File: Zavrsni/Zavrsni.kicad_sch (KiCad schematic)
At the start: 18 parts, among them J1 12V Source, J3 Output A, J4 Pin za Vin, J5 Conn_01x04, J6 Conn_02x19_Odd_Even, J7 Conn_02x19_Odd_Even, J8 Conn_01x06, U1 LM78M05_TO220, U2 L298N

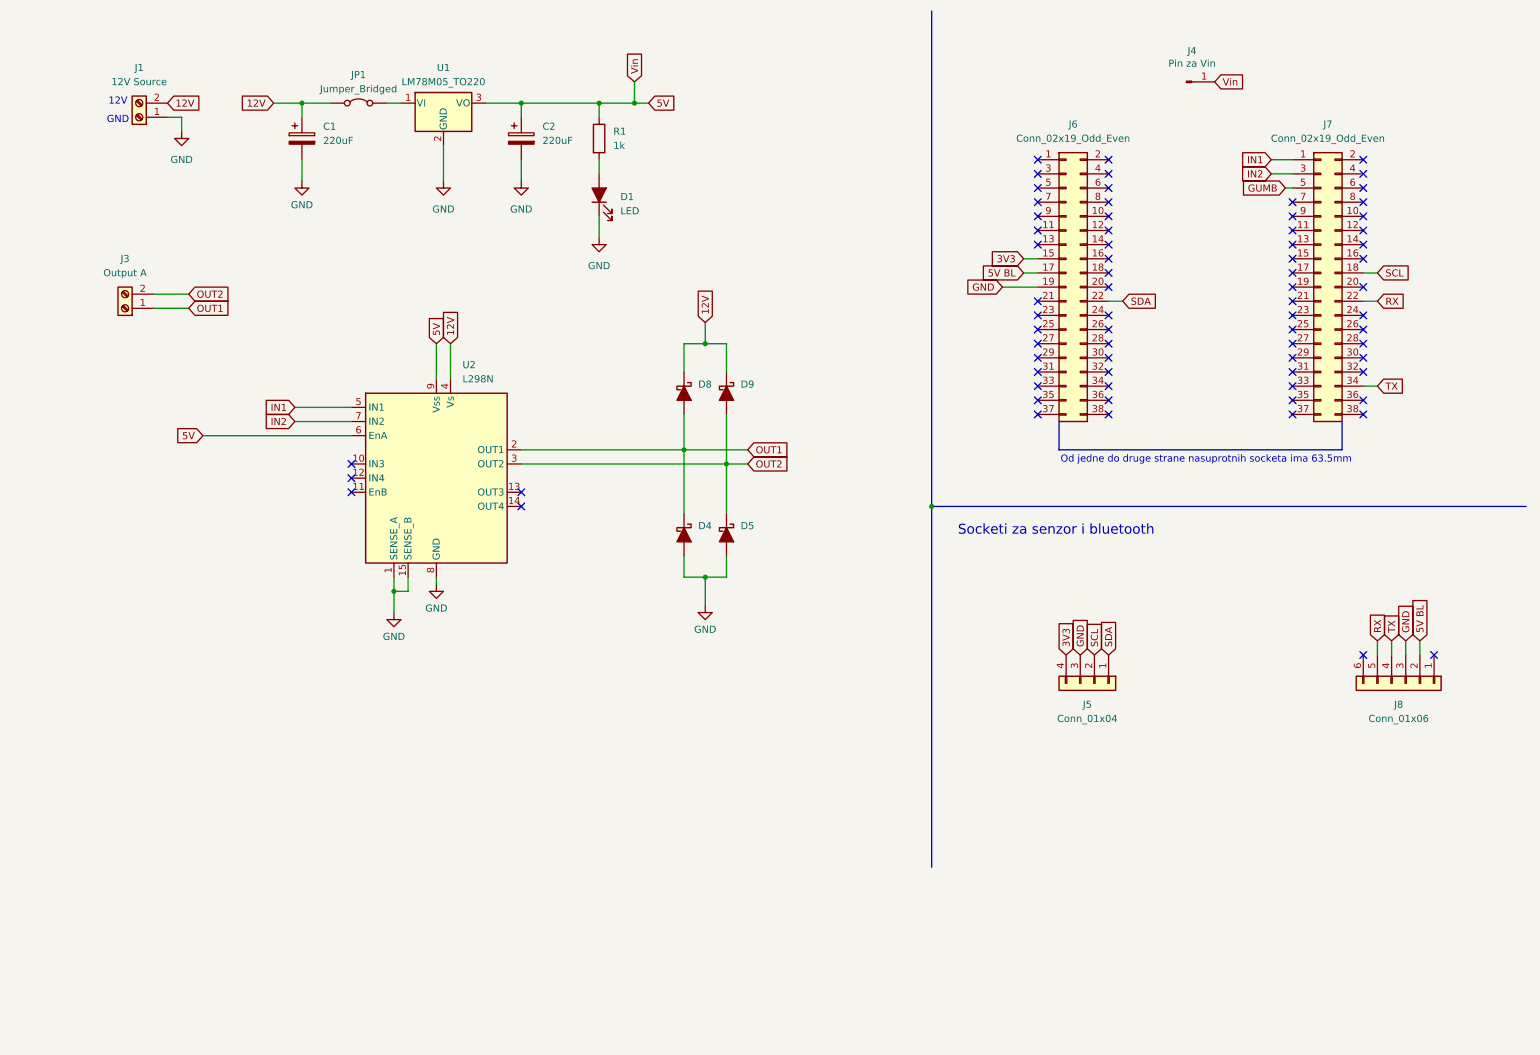
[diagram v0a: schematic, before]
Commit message: New
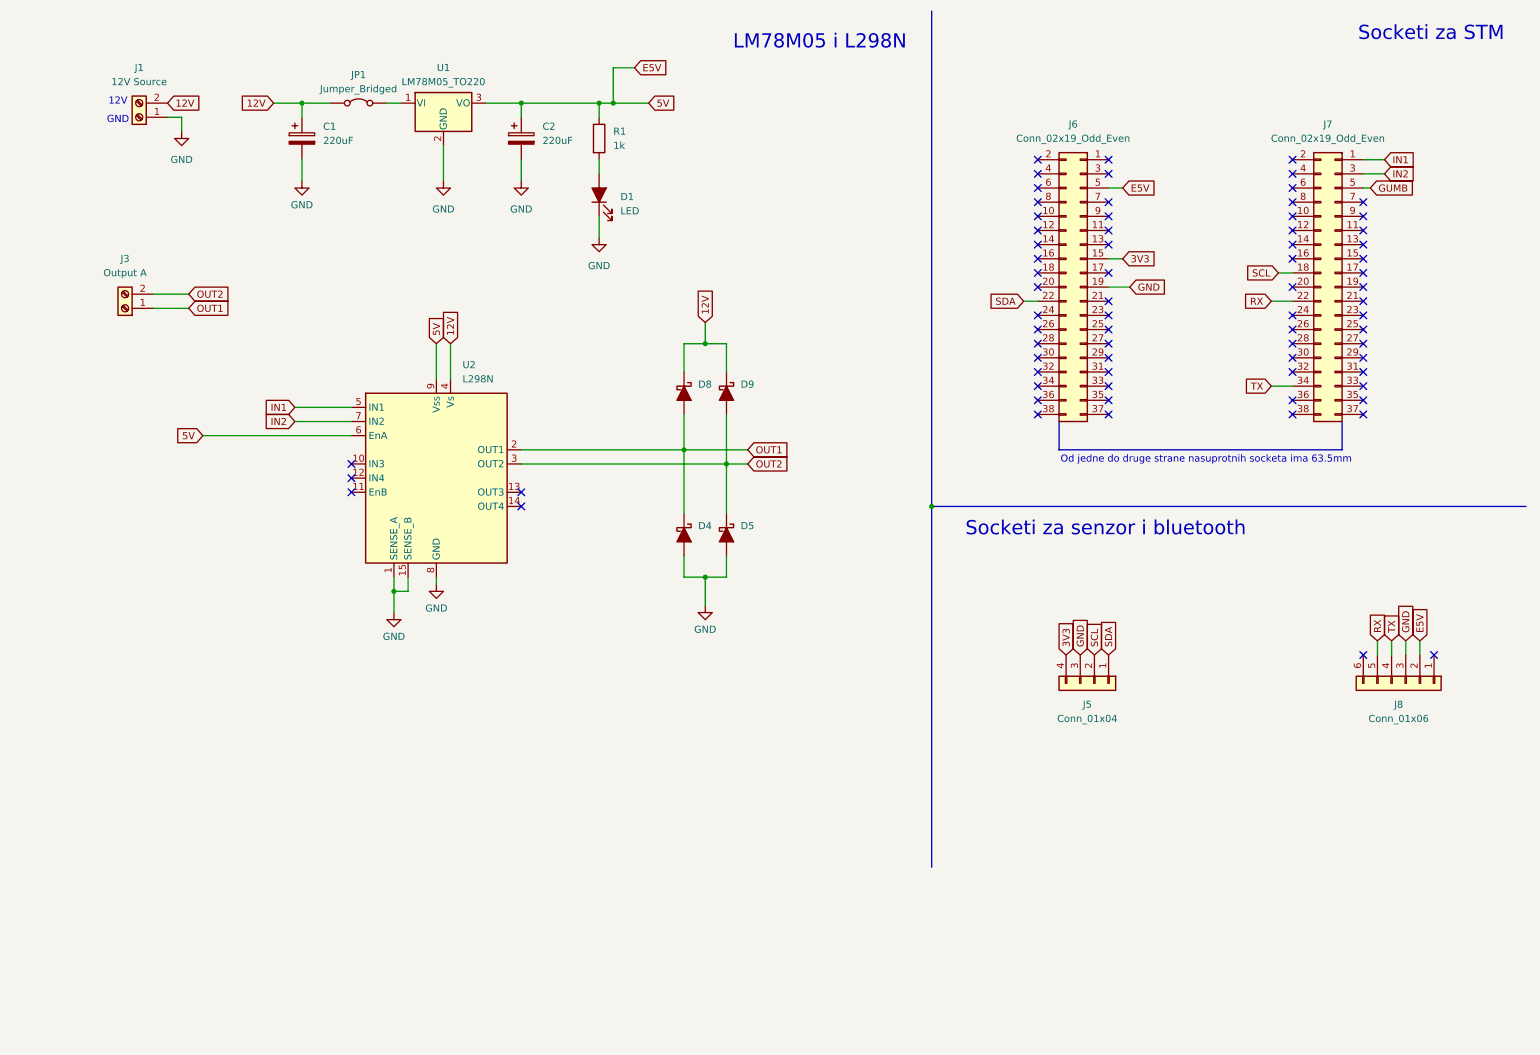
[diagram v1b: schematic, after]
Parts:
- removed J4: Pin za Vin, Connector_PinHeader_2.54mm:PinHeader_1x01_P2.54mm_Vertical, symbol Connector:Conn_01x01_Pin
- U1: Manufacturer (none) -> ONSEMI; Manufacturer part number (none) -> TO-220
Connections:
- net 5V: now also J6.5 (Pin_5), J8.2 (Pin_2)
- net 5V BL: no longer names the net of J6.17 (Pin_17)
- net 5V BL: no longer J8.2 (Pin_2)
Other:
- note added: "LM78M05 i L298N"
- note added: "Socketi za STM"

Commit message: New
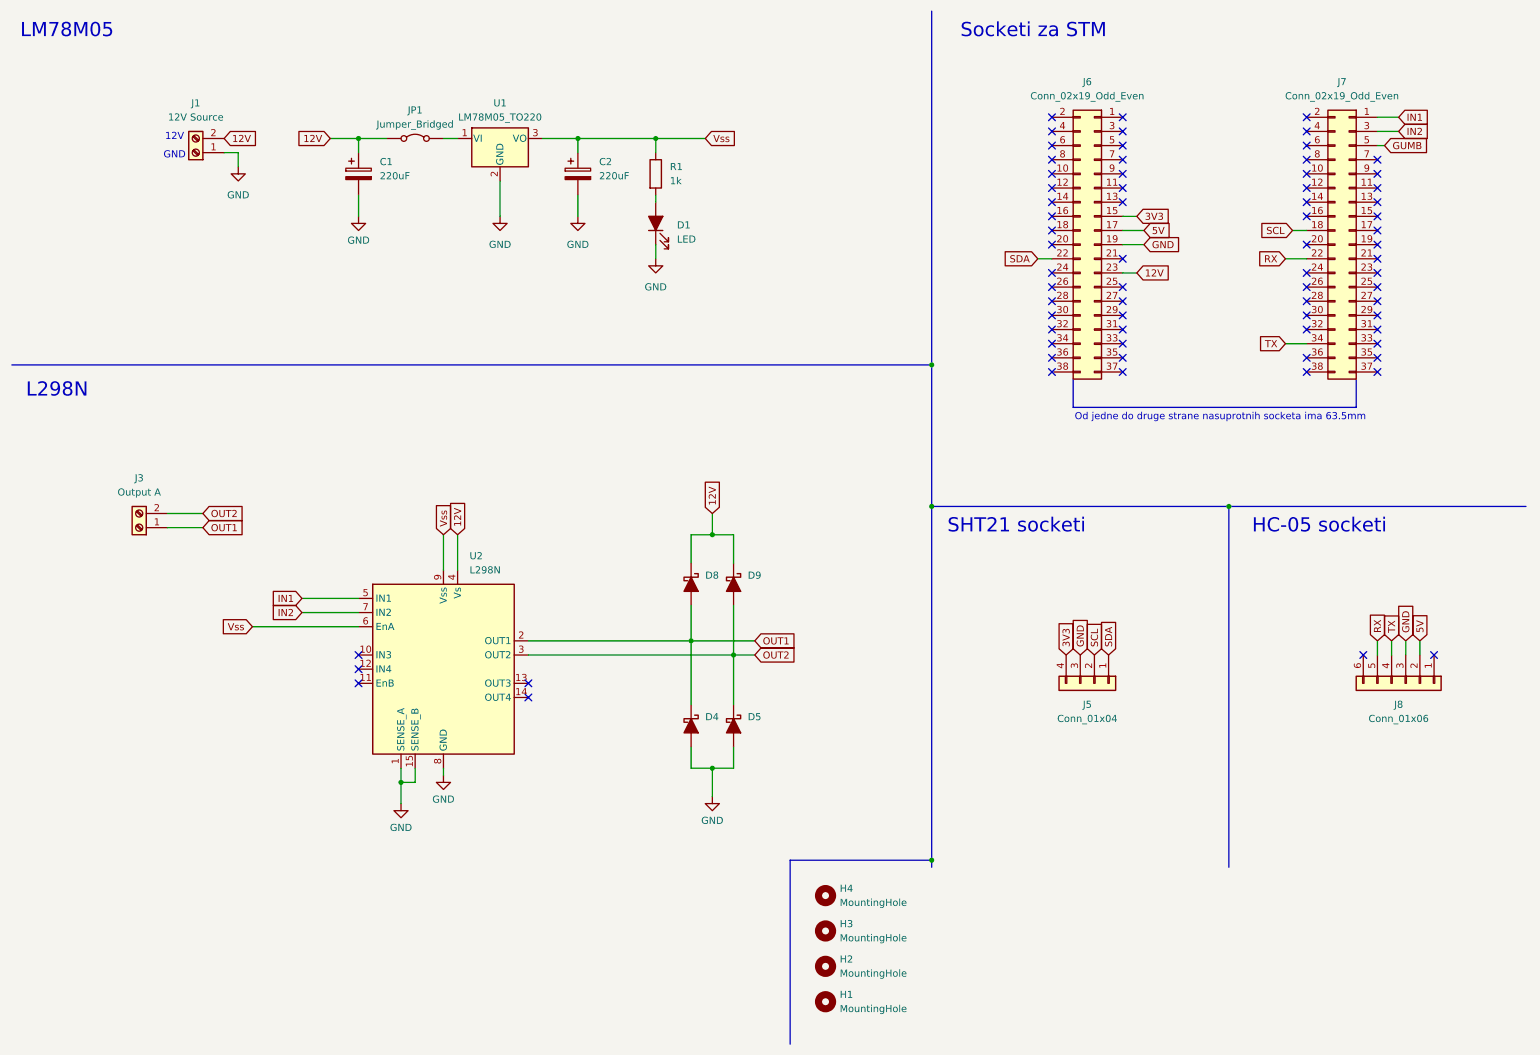
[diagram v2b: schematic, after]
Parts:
- added H1, H2, H3, H4: MountingHole, MountingHole:MountingHole_2.2mm_M2_ISO7380, symbol Mechanical:MountingHole
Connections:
- net 12V: now also J6.23 (Pin_23)
- net 5V: now also J6.17 (Pin_17); no longer C2.1, J6.5 (Pin_5), R1.1, U1.3 (VO), U2.6 (EnA), U2.9 (Vss)
- new net Vss: C2.1, R1.1, U1.3 (VO), U2.6 (EnA), U2.9 (Vss)
- no-connect marks 73 -> 72
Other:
- note added: "HC-05 socketi"
- note added: "L298N"
- note added: "LM78M05"
- note added: "SHT21 socketi"
- note removed: "LM78M05 i L298N"
- note removed: "Socketi za senzor i bluetooth"
- company: (none) -> TVZ
- title: (none) -> Zavrsni rad
- moved on the sheet: C1, C2, D1, D4, D5, D8, D9, J1, J3, J6, J7, JP1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

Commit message: New 4
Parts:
- H1, H2, H3, H4: footprint MountingHole:MountingHole_2.2mm_M2_ISO7380 -> MountingHole:MountingHole_3mm
- R1: footprint Resistor_SMD:R_1206_3216Metric_Pad1.30x1.75mm_HandSolder -> Resistor_THT:R_Axial_DIN0204_L3.6mm_D1.6mm_P5.08mm_Horizontal
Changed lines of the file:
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@@
 			)
 		)
-		(property "Footprint" "MountingHole:MountingHole_2.2mm_M2_ISO7380"
+		(property "Footprint" "MountingHole:MountingHole_3mm"
 			(at 158.75 190.5 0)
 			(effects
@@
 			)
 		)
-		(property "Footprint" "MountingHole:MountingHole_2.2mm_M2_ISO7380"
+		(property "Footprint" "MountingHole:MountingHole_3mm"
 			(at 158.75 171.45 0)
 			(effects
@@
 			)
 		)
-		(property "Footprint" "MountingHole:MountingHole_2.2mm_M2_ISO7380"
+		(property "Footprint" "MountingHole:MountingHole_3mm"
 			(at 158.75 177.8 0)
 			(effects
@@
 			)
 		)
-		(property "Footprint" "MountingHole:MountingHole_2.2mm_M2_ISO7380"
+		(property "Footprint" "MountingHole:MountingHole_3mm"
 			(at 158.75 184.15 0)
 			(effects
@@
 			)
 		)
-		(property "Footprint" "Resistor_SMD:R_1206_3216Metric_Pad1.30x1.75mm_HandSolder"
+		(property "Footprint" "Resistor_THT:R_Axial_DIN0204_L3.6mm_D1.6mm_P5.08mm_Horizontal"
 			(at 126.492 41.91 90)
 			(effects

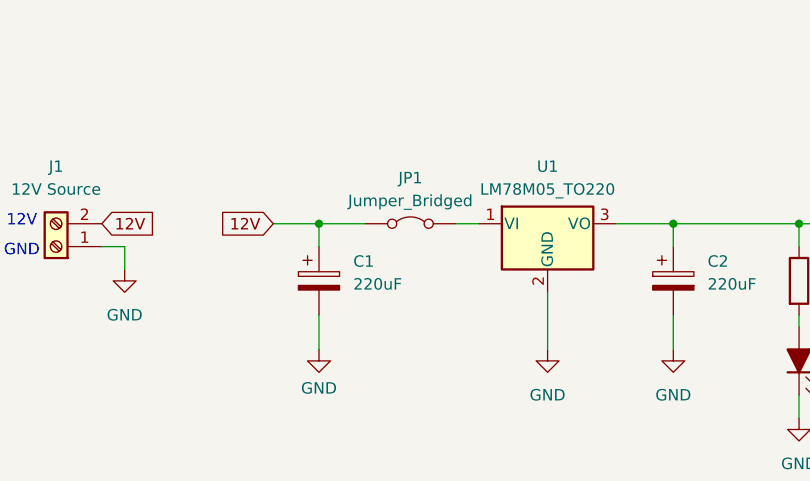
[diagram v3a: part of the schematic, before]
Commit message: Final
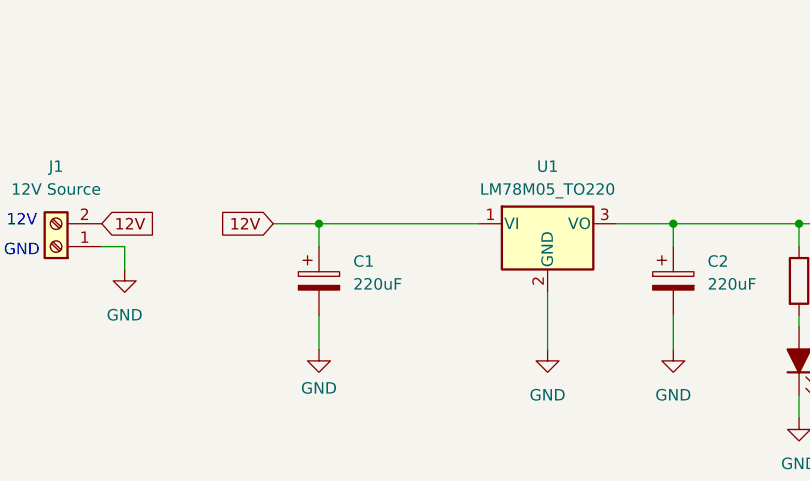
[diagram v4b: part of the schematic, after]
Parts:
- removed JP1: Jumper_Bridged, Connector_PinHeader_2.54mm:PinHeader_1x02_P2.54mm_Vertical, symbol Jumper:Jumper_2_Bridged
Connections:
- net 12V: now also U1.1 (VI)
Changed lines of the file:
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@@
 	(wire
 		(pts
-			(xy 74.93 35.56) (xy 80.01 35.56)
+			(xy 74.93 35.56) (xy 92.71 35.56)
 		)
 		(stroke
@@
 		(pts
 			(xy 82.55 148.59) (xy 82.55 151.13)
-		)
-		(stroke
-			(width 0)
-			(type default)
-		)
-	)
-	(wire
-		(pts
-			(xy 90.17 35.56) (xy 92.71 35.56)
 		)
 		(stroke
@@
 					(unit 1)
 				)
-			)
-		)
-	)
-	(symbol
-		(lib_id "Jumper:Jumper_2_Bridged")
-		(at 85.09 35.56 0)
-		(unit 1)
-		(exclude_from_sim no)
-		(in_bom yes)
-		(on_board yes)
-		(dnp no)
-		(fields_autoplaced yes)
-		(property "Reference" "JP1"
-			(at 85.09 30.48 0)
-			(effects
-				(font
-					(size 1.27 1.27)
-				)
-			)
-		)
-		(property "Value" "Jumper_Bridged"
-			(at 85.09 33.02 0)
-			(effects
-				(font
-					(size 1.27 1.27)
-				)
-			)
-		)
-		(property "Footprint" "Connector_PinHeader_2.54mm:PinHeader_1x02_P2.54mm_Vertical"
-			(at 85.09 35.56 0)
-			(effects
-				(font
-					(size 1.27 1.27)
-				)
-				(hide yes)
-			)
-		)
-		(property "Datasheet" "~"
-			(at 85.09 35.56 0)
-			(effects
-				(font
-					(size 1.27 1.27)
-				)
-				(hide yes)
-			)
-		)
-		(property "Description" "Jumper, 2-pole, closed/bridged"
-			(at 85.09 35.56 0)
-			(effects
-				(font
-					(size 1.27 1.27)
-				)
-				(hide yes)
-			)
-		)
-		(pin "1"
-		)
-		(pin "2"
-		)
-		(instances
-			(project ""
-				(path "/f2ac0668-a3c8-4093-af03-acd91b31ec7e"
-					(reference "JP1")
-					(unit 1)
-				)
